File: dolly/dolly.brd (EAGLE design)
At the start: 31 parts, among them U1 ATTINY85-20P

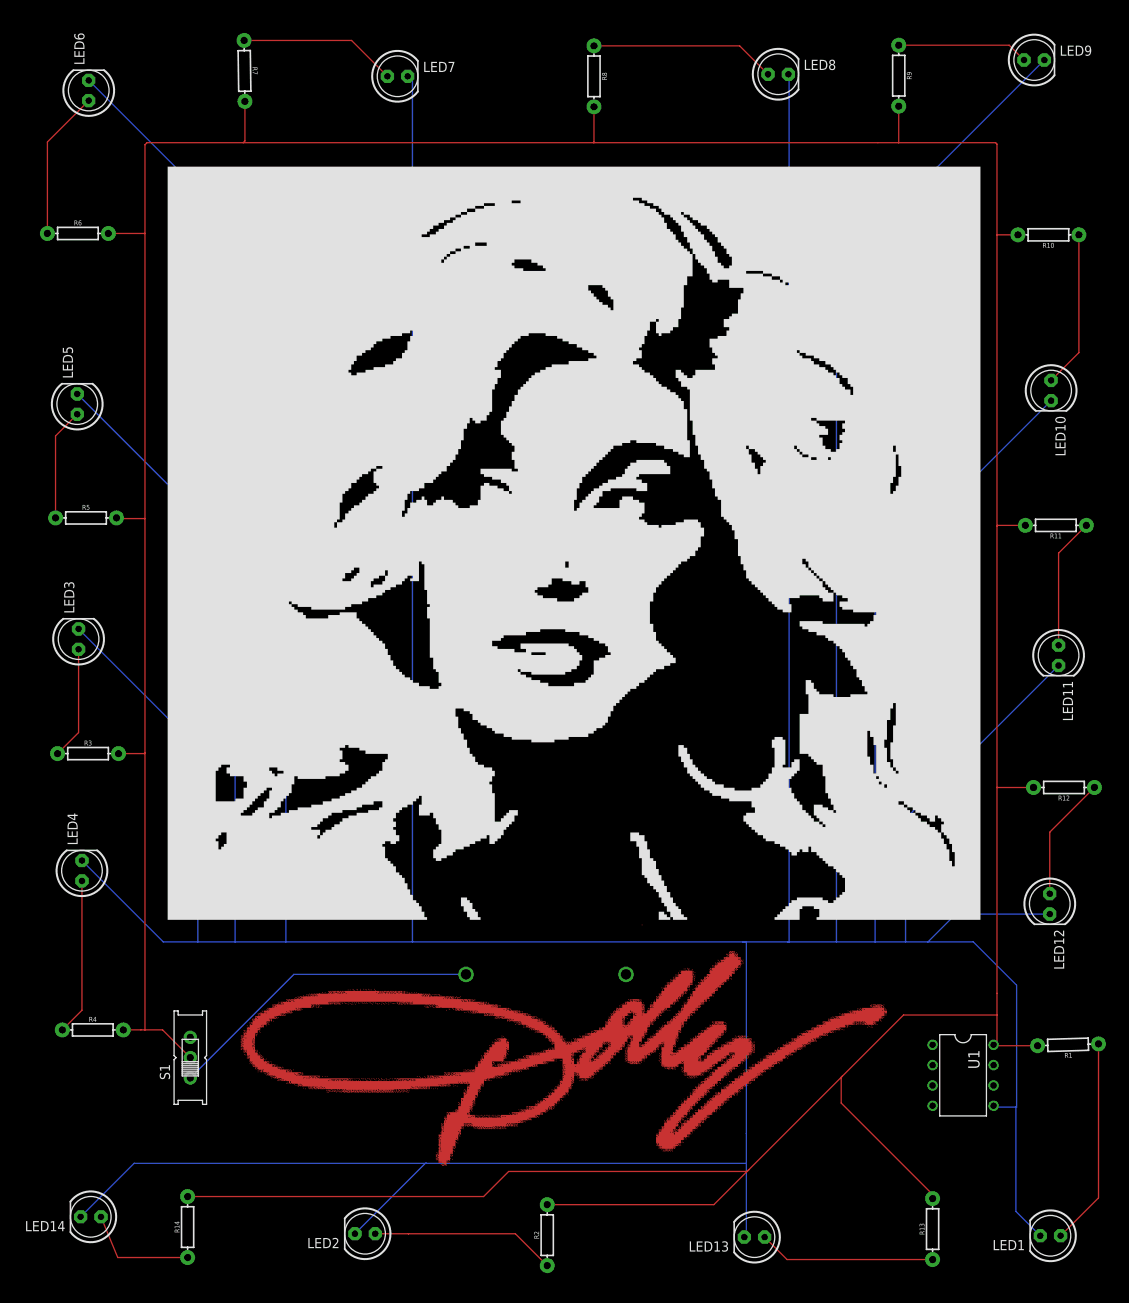
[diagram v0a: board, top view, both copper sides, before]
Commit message: DOLLY BADGE OK LOL
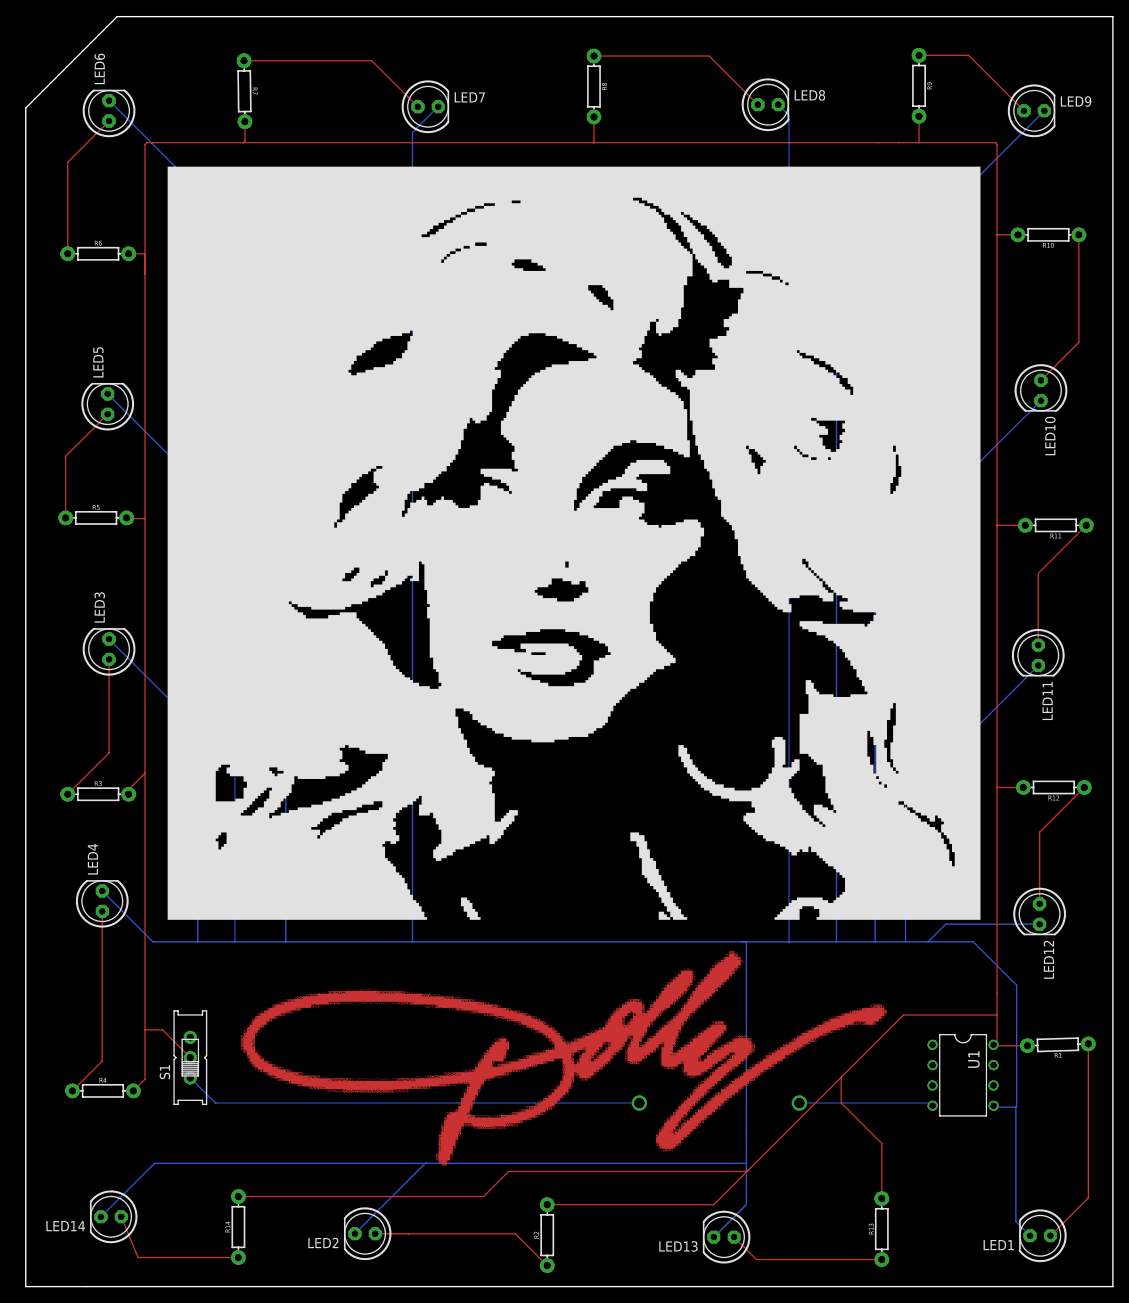
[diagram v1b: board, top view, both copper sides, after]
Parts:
- moved BT1 27.0 mm to (70.8, 10.2)
- moved R4 7.73 mm to (-8.13, 11.8)
- moved R13 6.35 mm to (89.2, -5.51)
- moved R14 6.35 mm to (8.80, -5.25)
- moved LED9 6.35 mm to (108.3, 134.3)
- moved LED7 5.39 mm to (32.5, 134.8)
- moved R3 5.24 mm to (-8.72, 48.8)
- moved LED4 4.58 mm to (-8.22, 35.5)
- moved LED8 4.02 mm to (75.0, 135.0)
- moved LED3 4.02 mm to (-7.37, 67.0)
- moved LED5 3.81 mm to (-7.54, 97.6)
- moved LED13 3.81 mm to (69.5, -6.52)
- moved LED6 3.59 mm to (-7.37, 134.3)
- moved R6 3.59 mm to (-8.72, 116.4)
- moved R9 2.84 mm to (93.9, 137.4)
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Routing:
- net N$4: track 1014.2 -> 987.9 mm
- net N$2: track 39.8 -> 58.1 mm
- net N$5: track 0.00 -> 17.3 mm
- net N$6: track 540.1 -> 527.8 mm
- net N$3: track 14.1 -> 19.0 mm
- net N$10: track 19.8 -> 24.1 mm
- net N$7: track 19.6 -> 24.0 mm
- net N$17: track 14.2 -> 18.0 mm
- net N$16: track 22.2 -> 19.6 mm
- net N$15: track 15.6 -> 16.9 mm
- net N$14: track 16.4 -> 17.5 mm
- net N$8: track 14.1 -> 15.1 mm
- net N$13: track 19.6 -> 20.2 mm
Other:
- board outline added: 135.9 x 158.8 mm

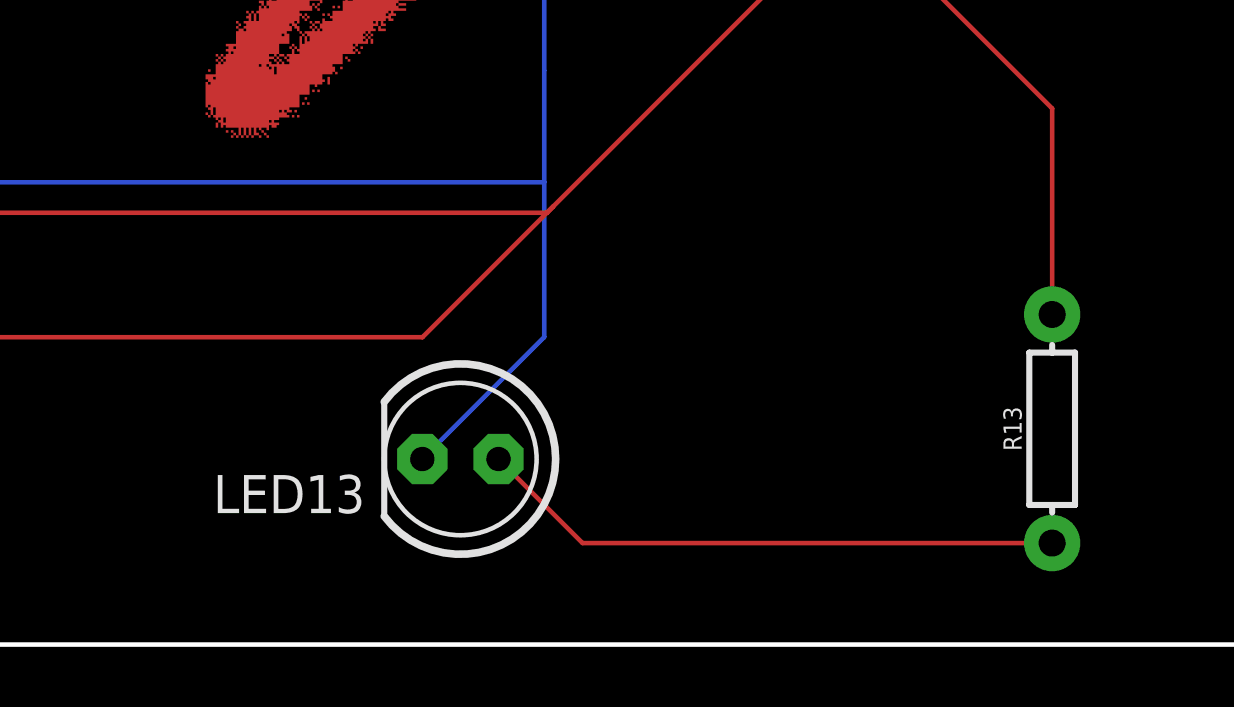
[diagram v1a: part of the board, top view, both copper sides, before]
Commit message: DOLLY BADGE OK LOL
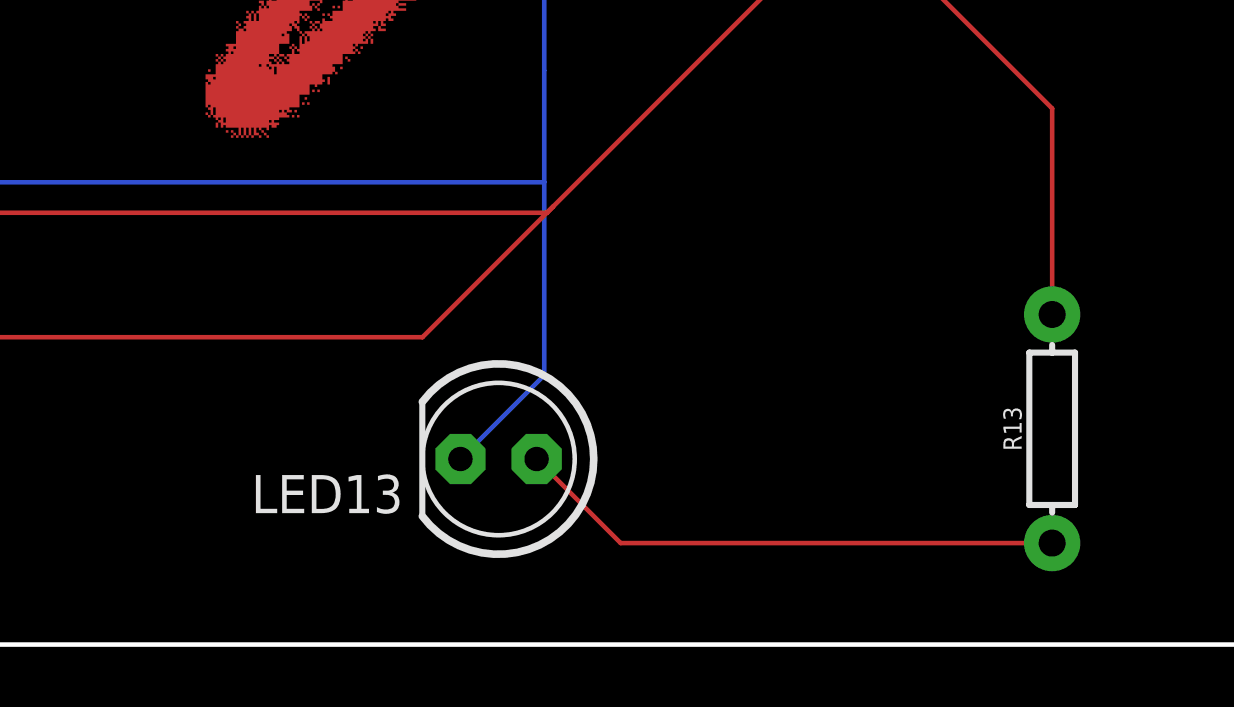
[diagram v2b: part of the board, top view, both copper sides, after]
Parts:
- moved LED13 1.27 mm to (70.8, -6.52)
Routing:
- net N$16: track 19.6 -> 18.3 mm
- net N$4: track 987.9 -> 987.3 mm
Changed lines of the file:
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@@
 <element name="LED11" library="adafruit" package="LED5MM" value="" x="108.781978125" y="66.206140625" rot="R270"/>
 <element name="LED12" library="adafruit" package="LED5MM" value="" x="108.951421875" y="33.865825" rot="R270"/>
-<element name="LED13" library="adafruit" package="LED5MM" value="" x="69.49918125" y="-6.516009375" rot="R180"/>
+<element name="LED13" library="adafruit" package="LED5MM" value="" x="70.76918125" y="-6.516009375" rot="R180"/>
 <element name="LED14" library="adafruit" package="LED5MM" value="" x="-7.113321875" y="-3.975503125" rot="R180"/>
 <element name="LED2" library="adafruit" package="LED5MM" value="" x="24.633371875" y="-6.091196875" rot="R180"/>
@@
 <wire x1="72.293159375" y1="6.434021875" x2="72.293159375" y2="30.39229375" width="0.1524" layer="16"/>
 <wire x1="71.874809375" y1="30.39229375" x2="71.95946875" y2="30.39229375" width="0.1524" layer="16"/>
-<wire x1="68.22918125" y1="-6.516009375" x2="72.293159375" y2="-2.45203125" width="0.1524" layer="16"/>
+<wire x1="69.49918125" y1="-6.516009375" x2="72.293159375" y2="-3.72203125" width="0.1524" layer="16"/>
 <wire x1="71.874809375" y1="30.39229375" x2="77.46225" y2="30.39229375" width="0.1524" layer="16"/>
 <wire x1="23.363371875" y1="-6.091196875" x2="32.16363125" y2="2.7090625" width="0.1524" layer="16"/>
 <wire x1="32.16363125" y1="2.7090625" x2="32.33943125" y2="2.7090625" width="0.1524" layer="16"/>
 <wire x1="32.33943125" y1="2.7090625" x2="72.293159375" y2="2.7090625" width="0.1524" layer="16"/>
-<wire x1="72.293159375" y1="-2.45203125" x2="72.293159375" y2="2.7090625" width="0.1524" layer="16"/>
+<wire x1="72.293159375" y1="-3.72203125" x2="72.293159375" y2="2.7090625" width="0.1524" layer="16"/>
 <wire x1="-8.383321875" y1="-3.975503125" x2="-1.69875625" y2="2.7090625" width="0.1524" layer="16"/>
 <wire x1="-1.69875625" y1="2.7090625" x2="32.33943125" y2="2.7090625" width="0.1524" layer="16"/>
@@
 <contactref element="R13" pad="P$1"/>
 <contactref element="LED13" pad="A"/>
-<wire x1="89.22415625" y1="-9.317609375" x2="73.57078125" y2="-9.317609375" width="0.1524" layer="1"/>
-<wire x1="73.57078125" y1="-9.317609375" x2="70.76918125" y2="-6.516009375" width="0.1524" layer="1"/>
+<wire x1="89.22415625" y1="-9.317609375" x2="74.84078125" y2="-9.317609375" width="0.1524" layer="1"/>
+<wire x1="74.84078125" y1="-9.317609375" x2="72.03918125" y2="-6.516009375" width="0.1524" layer="1"/>
 </signal>
 <signal name="N$17">

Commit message: DOLLY BADGE OK LOL
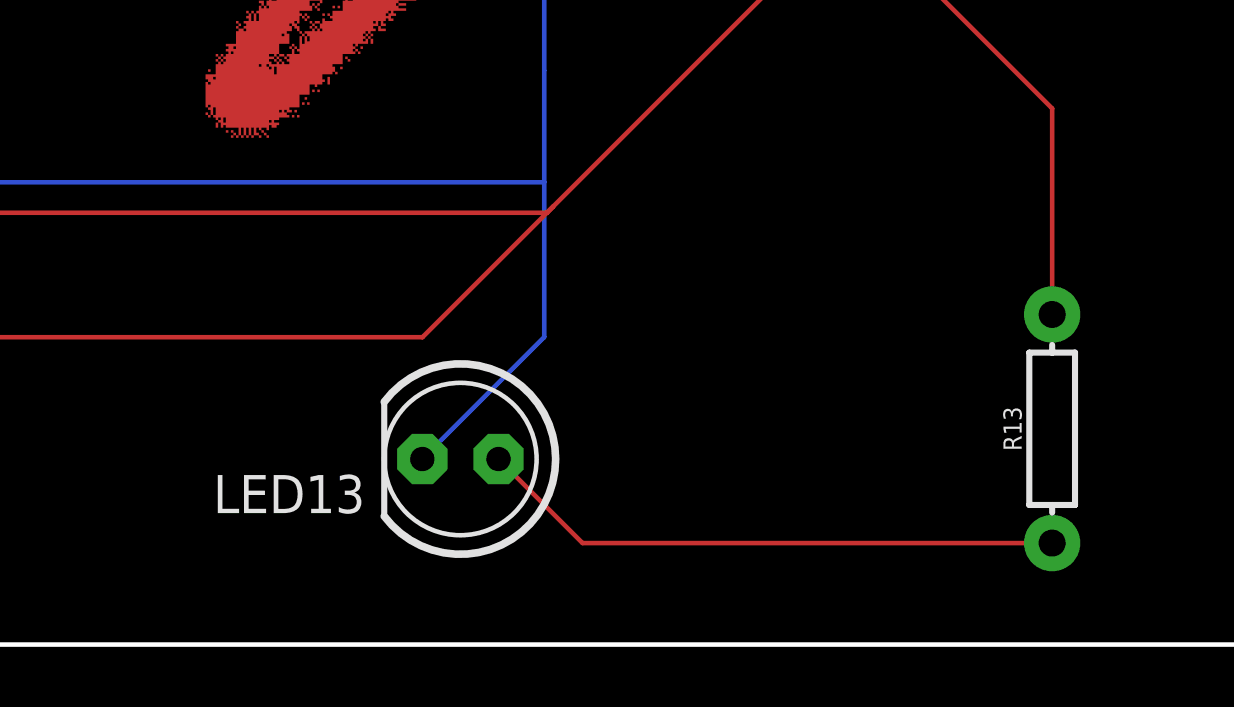
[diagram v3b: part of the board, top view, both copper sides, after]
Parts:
- moved LED13 1.27 mm to (69.5, -6.52)
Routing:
- net N$16: track 18.3 -> 19.6 mm
- net N$4: track 987.3 -> 987.9 mm
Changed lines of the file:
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@@
 <element name="LED11" library="adafruit" package="LED5MM" value="" x="108.781978125" y="66.206140625" rot="R270"/>
 <element name="LED12" library="adafruit" package="LED5MM" value="" x="108.951421875" y="33.865825" rot="R270"/>
-<element name="LED13" library="adafruit" package="LED5MM" value="" x="70.76918125" y="-6.516009375" rot="R180"/>
+<element name="LED13" library="adafruit" package="LED5MM" value="" x="69.49918125" y="-6.516009375" rot="R180"/>
 <element name="LED14" library="adafruit" package="LED5MM" value="" x="-7.113321875" y="-3.975503125" rot="R180"/>
 <element name="LED2" library="adafruit" package="LED5MM" value="" x="24.633371875" y="-6.091196875" rot="R180"/>
@@
 <wire x1="72.293159375" y1="6.434021875" x2="72.293159375" y2="30.39229375" width="0.1524" layer="16"/>
 <wire x1="71.874809375" y1="30.39229375" x2="71.95946875" y2="30.39229375" width="0.1524" layer="16"/>
-<wire x1="69.49918125" y1="-6.516009375" x2="72.293159375" y2="-3.72203125" width="0.1524" layer="16"/>
+<wire x1="68.22918125" y1="-6.516009375" x2="72.293159375" y2="-2.45203125" width="0.1524" layer="16"/>
 <wire x1="71.874809375" y1="30.39229375" x2="77.46225" y2="30.39229375" width="0.1524" layer="16"/>
 <wire x1="23.363371875" y1="-6.091196875" x2="32.16363125" y2="2.7090625" width="0.1524" layer="16"/>
 <wire x1="32.16363125" y1="2.7090625" x2="32.33943125" y2="2.7090625" width="0.1524" layer="16"/>
 <wire x1="32.33943125" y1="2.7090625" x2="72.293159375" y2="2.7090625" width="0.1524" layer="16"/>
-<wire x1="72.293159375" y1="-3.72203125" x2="72.293159375" y2="2.7090625" width="0.1524" layer="16"/>
+<wire x1="72.293159375" y1="-2.45203125" x2="72.293159375" y2="2.7090625" width="0.1524" layer="16"/>
 <wire x1="-8.383321875" y1="-3.975503125" x2="-1.69875625" y2="2.7090625" width="0.1524" layer="16"/>
 <wire x1="-1.69875625" y1="2.7090625" x2="32.33943125" y2="2.7090625" width="0.1524" layer="16"/>
@@
 <contactref element="R13" pad="P$1"/>
 <contactref element="LED13" pad="A"/>
-<wire x1="89.22415625" y1="-9.317609375" x2="74.84078125" y2="-9.317609375" width="0.1524" layer="1"/>
-<wire x1="74.84078125" y1="-9.317609375" x2="72.03918125" y2="-6.516009375" width="0.1524" layer="1"/>
+<wire x1="89.22415625" y1="-9.317609375" x2="73.57078125" y2="-9.317609375" width="0.1524" layer="1"/>
+<wire x1="73.57078125" y1="-9.317609375" x2="70.76918125" y2="-6.516009375" width="0.1524" layer="1"/>
 </signal>
 <signal name="N$17">
